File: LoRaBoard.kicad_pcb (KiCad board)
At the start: 2 copper layers, 20 parts, among them J1 Prog, J2 I2C, J3 UART, J4 GPIO, J5 ADC/SPI, J6 CONN_01X02, J7 PWR, SW1 RESET, U1 im880b, U2 LDO-TPS78233, X1 SMACONNECTOR

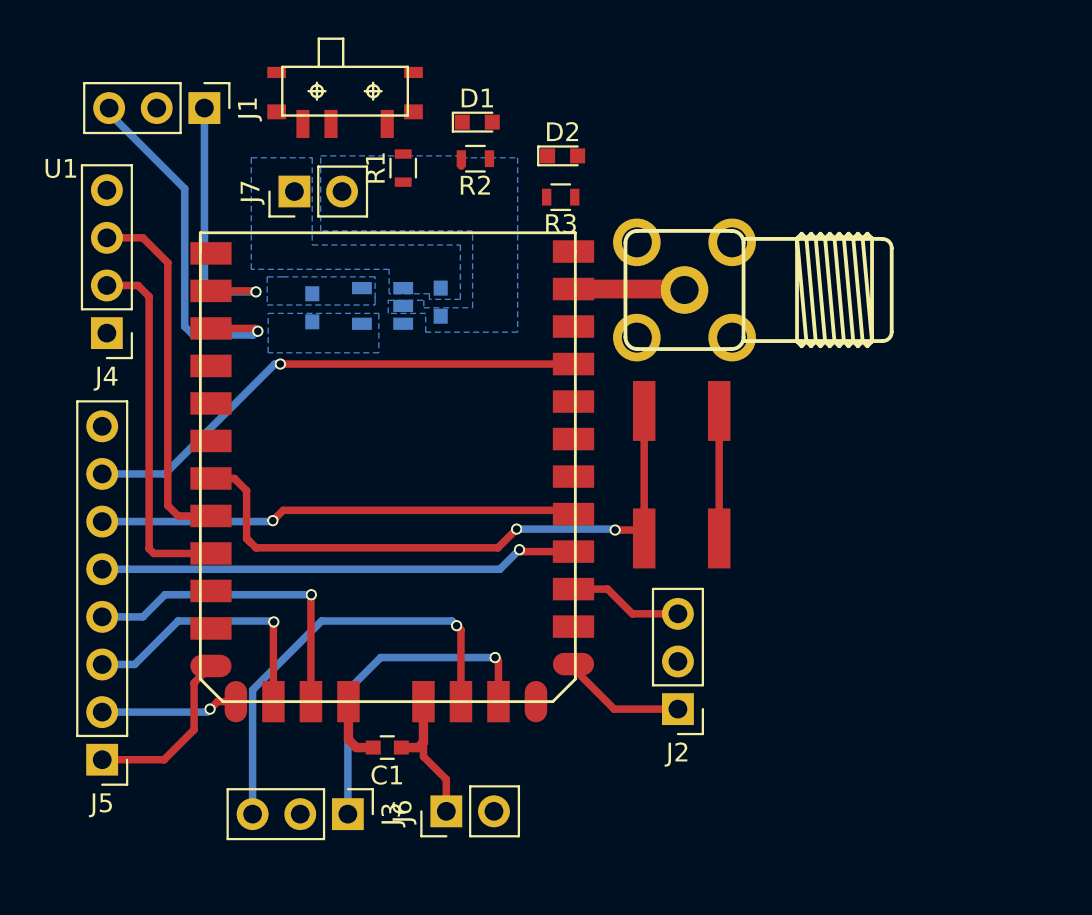
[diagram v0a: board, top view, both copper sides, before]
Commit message: LoRaBoard Done
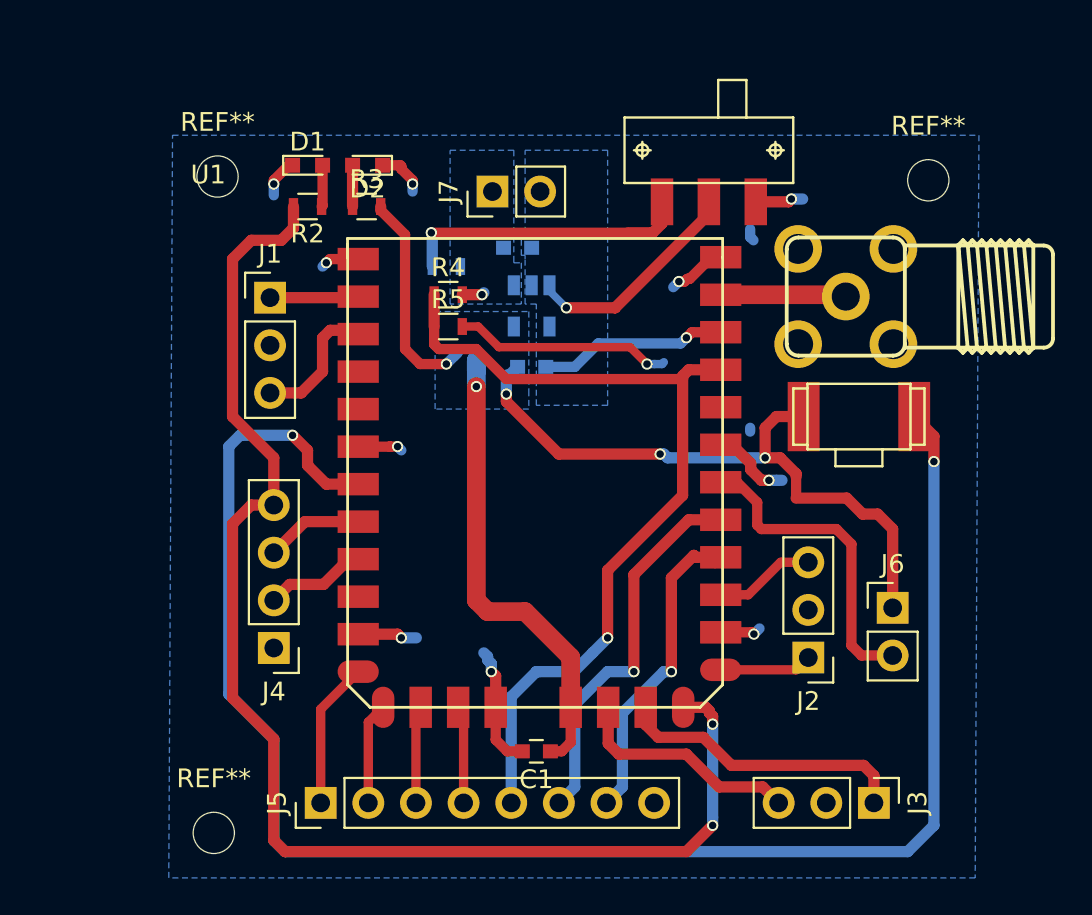
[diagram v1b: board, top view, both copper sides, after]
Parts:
- added R4: 33k, Resistors_SMD:R_0603, F.Cu at (153.3, 106.9)
- added R5: 10k, Resistors_SMD:R_0603, F.Cu at (153.3, 108.6)
- added REF**: MountingHole_2.2mm_M2_DIN965, Mounting_Holes:MountingHole_2.2mm_M2_DIN965, F.Cu at (178.9, 100.8)
- added REF**: MountingHole_2.2mm_M2_DIN965, Mounting_Holes:MountingHole_2.2mm_M2_DIN965, F.Cu at (140.8, 135.6)
- added REF**: MountingHole_2.2mm_M2_DIN965, Mounting_Holes:MountingHole_2.2mm_M2_DIN965, F.Cu at (141.0, 100.6)
- R1: moved to B.Cu
- S1: footprint SparkFun-Electromechanical:SWITCH-SPST-SMD-A -> SparkFun-Electromechanical:SWITCH-SPDT-SMD
- SW1: value RESET -> SWITCH_PUSHBUTTONC&K_KSS; footprint adafruit:EVQ-Q2 -> BTN_CK_KSS
- moved J3 28.1 mm to (176.0, 134.0)
- moved J6 26.2 mm to (177.0, 123.6), turned to 0 degrees
- moved S1 19.7 mm to (167.2, 99.2)
- moved J4 19.0 mm to (144.0, 125.7)
- moved C3 12.1 mm to (157.8, 110.8), turned to 0 degrees
- moved J5 11.9 mm to (146.5, 134.0), turned to 90 degrees
- moved J1 10.7 mm to (143.8, 107.1), turned to 0 degrees
- moved J7 10.6 mm to (155.7, 101.4)
- moved D2 10.4 mm to (149.0, 100.0), turned to 180 degrees
- moved R3 10.4 mm to (148.9, 102.2), turned to 0 degrees
- moved SW1 9.95 mm to (175.2, 113.4), turned to 0 degrees
- moved D1 9.34 mm to (145.8, 100.0)
- moved R2 9.31 mm to (145.8, 102.2)
- moved X1 8.61 mm to (174.5, 107.0)
- moved C1 7.95 mm to (158.0, 131.2)
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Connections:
- J5 pad 5: /P14 -> /P17
- J5 pad 7: /P17 -> /P14
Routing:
- net /P11: track 0.40 -> 71.4 mm, vias 0 -> 2
- net +3V3: track 14.4 -> 72.1 mm, vias 0 -> 5
- net /RESET: track 33.8 -> 89.0 mm
- net GND: track 3.52 -> 53.6 mm, vias 0 -> 12
- net /P17: track 27.6 -> 47.2 mm
- net /BOOT: track 0.00 -> 16.9 mm
- net Net-(R1-Pad2): track 0.00 -> 15.5 mm, vias 0 -> 1
- net /P5: track 19.3 -> 5.19 mm
- net /P6: track 19.3 -> 5.41 mm
- net /JTMS: track 20.1 -> 7.22 mm, vias 1 -> 0
- net /P10: track 17.3 -> 5.22 mm, vias 1 -> 0
- net /EN: track 0.00 -> 11.9 mm, vias 0 -> 1
- net /RXD: track 23.4 -> 12.3 mm, vias 1 -> 0
- net /JTCK: track 14.8 -> 4.72 mm, vias 1 -> 0
- net /P9: track 14.4 -> 5.20 mm, vias 1 -> 0
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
